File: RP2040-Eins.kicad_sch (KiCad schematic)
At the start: 55 parts, among them J1 Barrel_Jack_Switch, J10 USB_C_Receptacle_USB2.0, J2 CONN_I, J3 CONN_A, J4 CONN_P, J5 CONN_X, J7 CONN_JTAG, J8 CONN_D1, J9 CONN_D2, Q1 AO3401A, SW1 BOOTSEL, SW2 RESET, U1 W25Q128JVS, U2 RP2040, U3 AMS1117-5.0, U4 W25Q128JVEIQ, U5 AMS1117-3.3, U6 LM358, Y1 12MHz

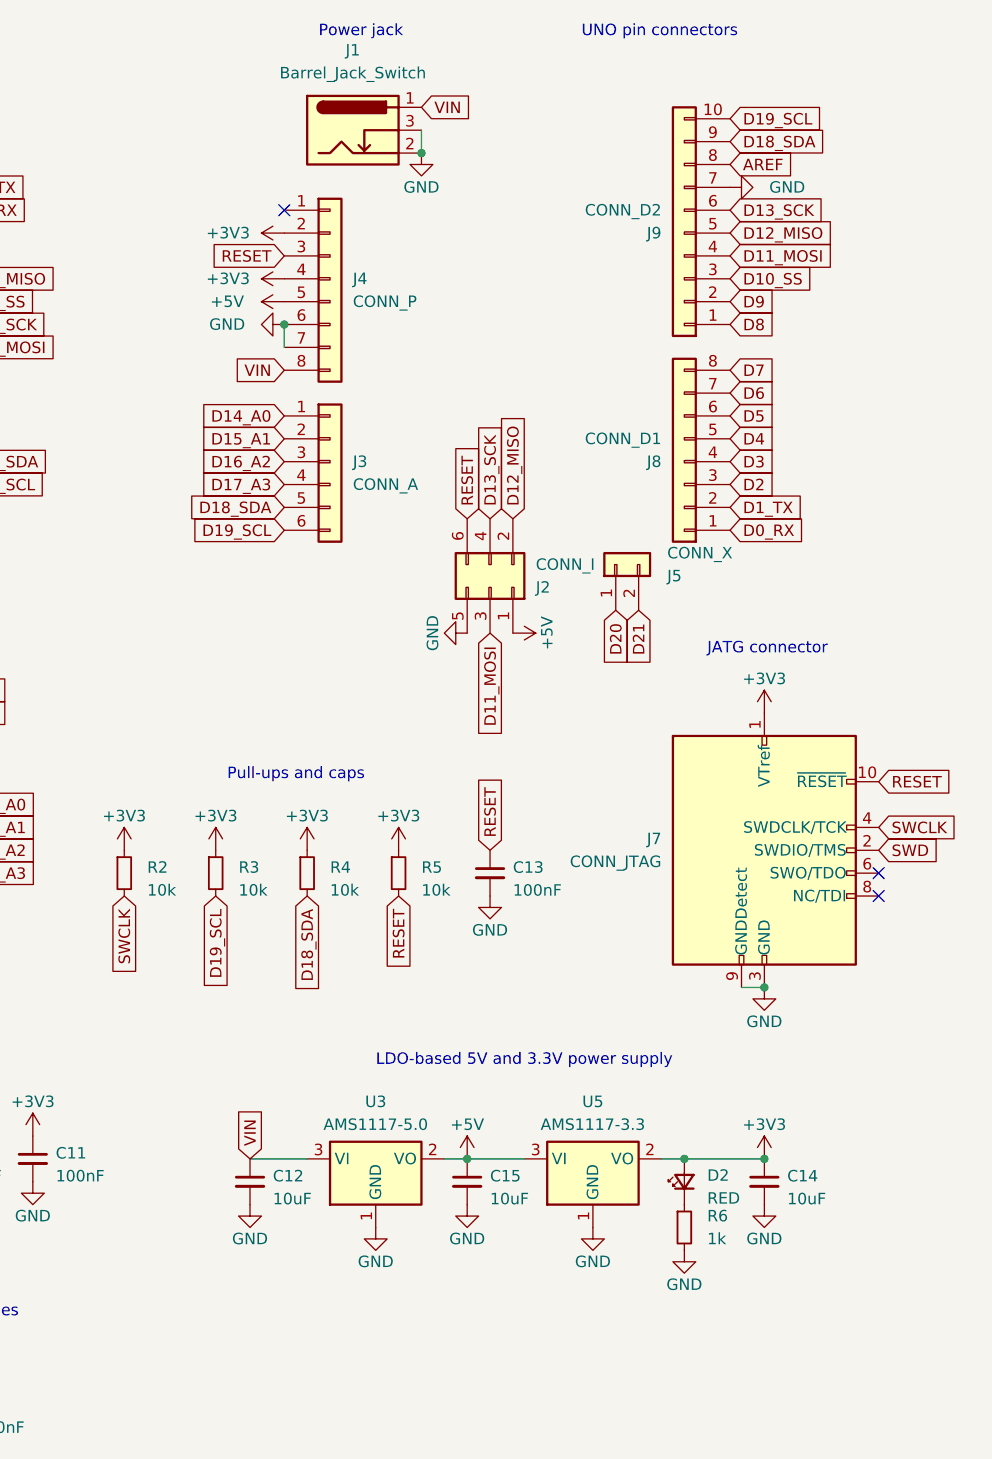
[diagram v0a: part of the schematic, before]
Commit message: Moved stuff around
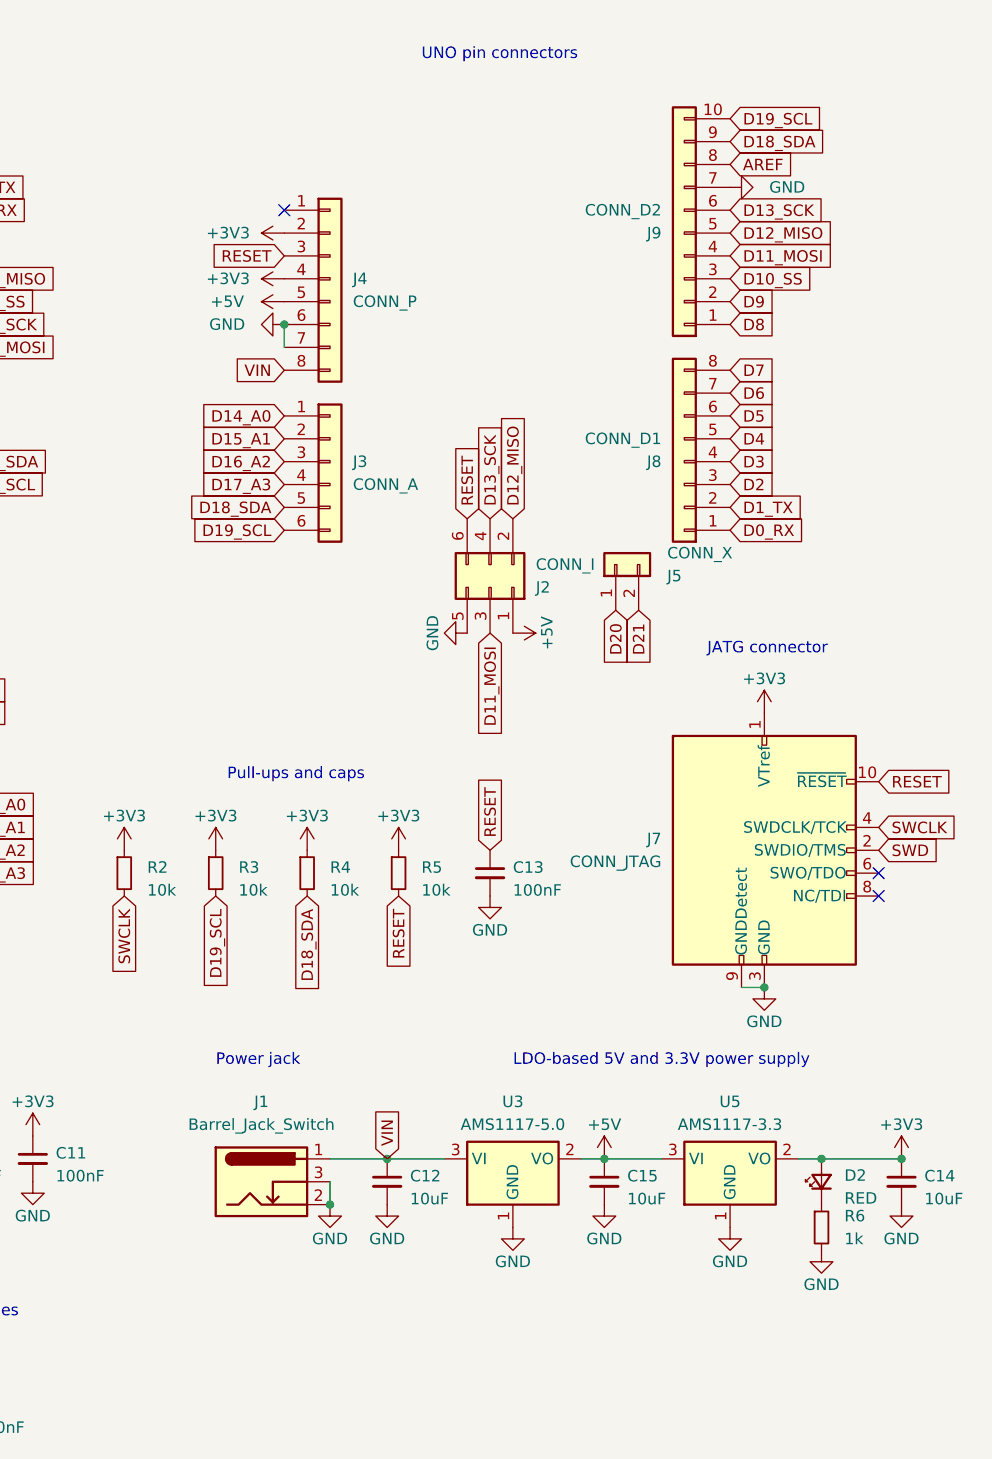
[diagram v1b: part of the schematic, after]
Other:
- moved on the sheet: C12, C14, C15, D2, J1, R6, U3, U5
